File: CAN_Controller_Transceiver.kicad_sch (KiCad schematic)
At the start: 31 parts, among them J11 Screw_Terminal_01x02, J12 DB9_Male, SW1 SW_SPDT, U1 MCP2515-xSO, U2 MCP2551-I-SN, U3 LD1117S50TR_SOT223, Y1 8MHz Crystal

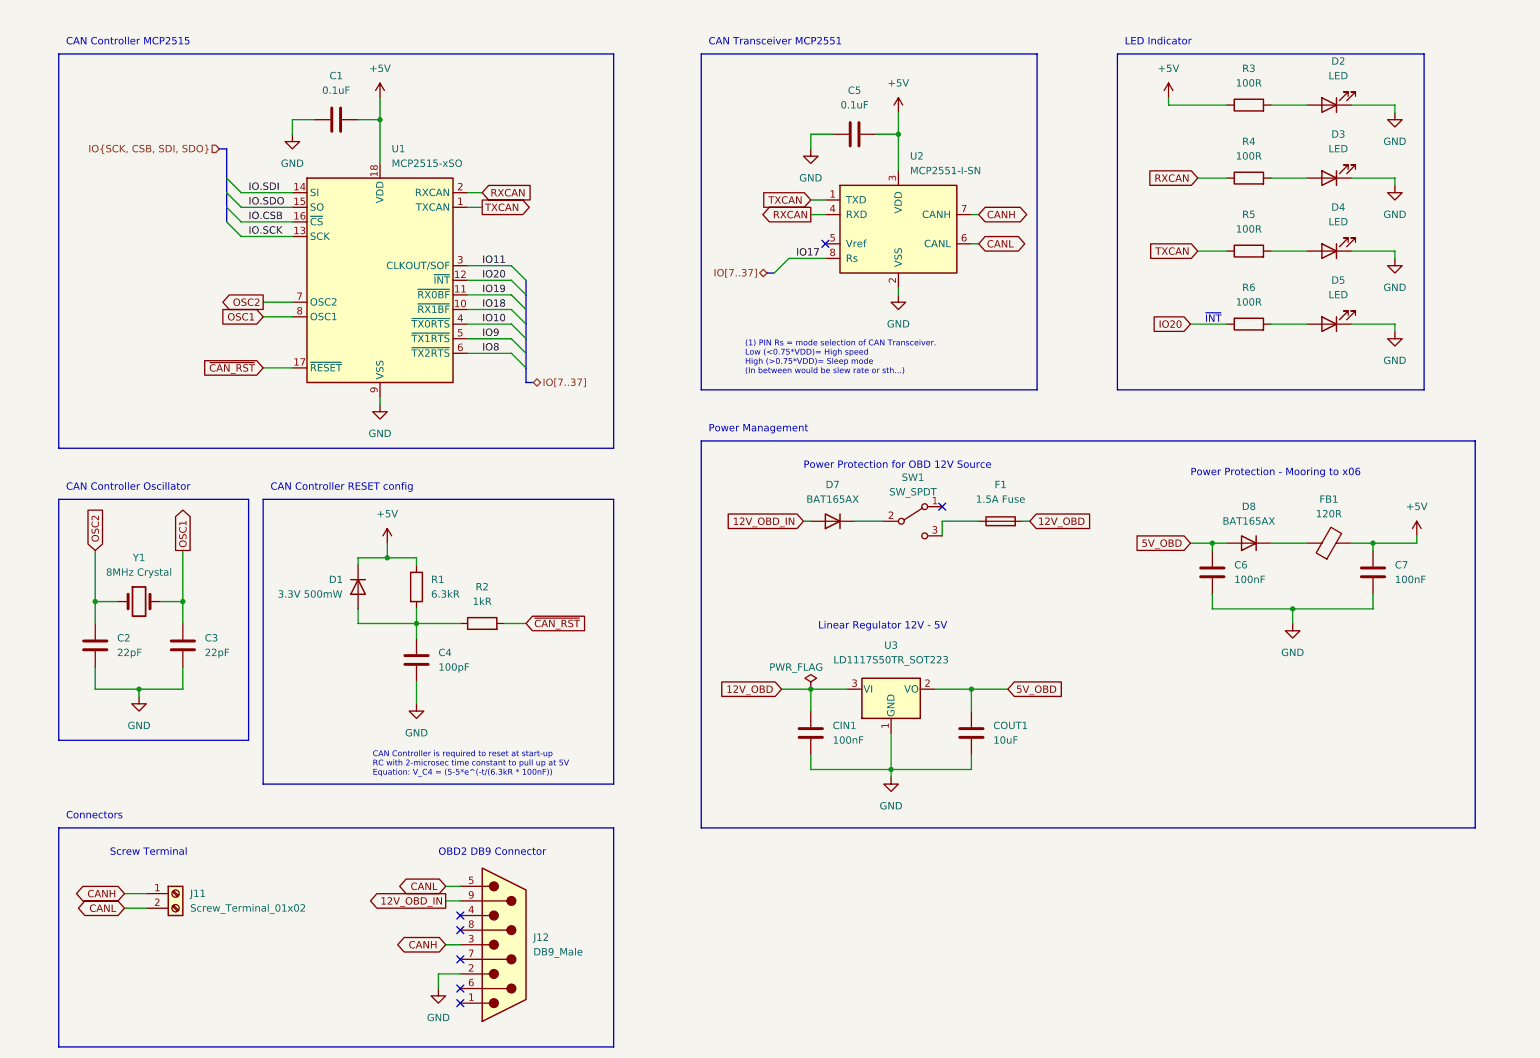
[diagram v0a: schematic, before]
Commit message: Complete board (1)
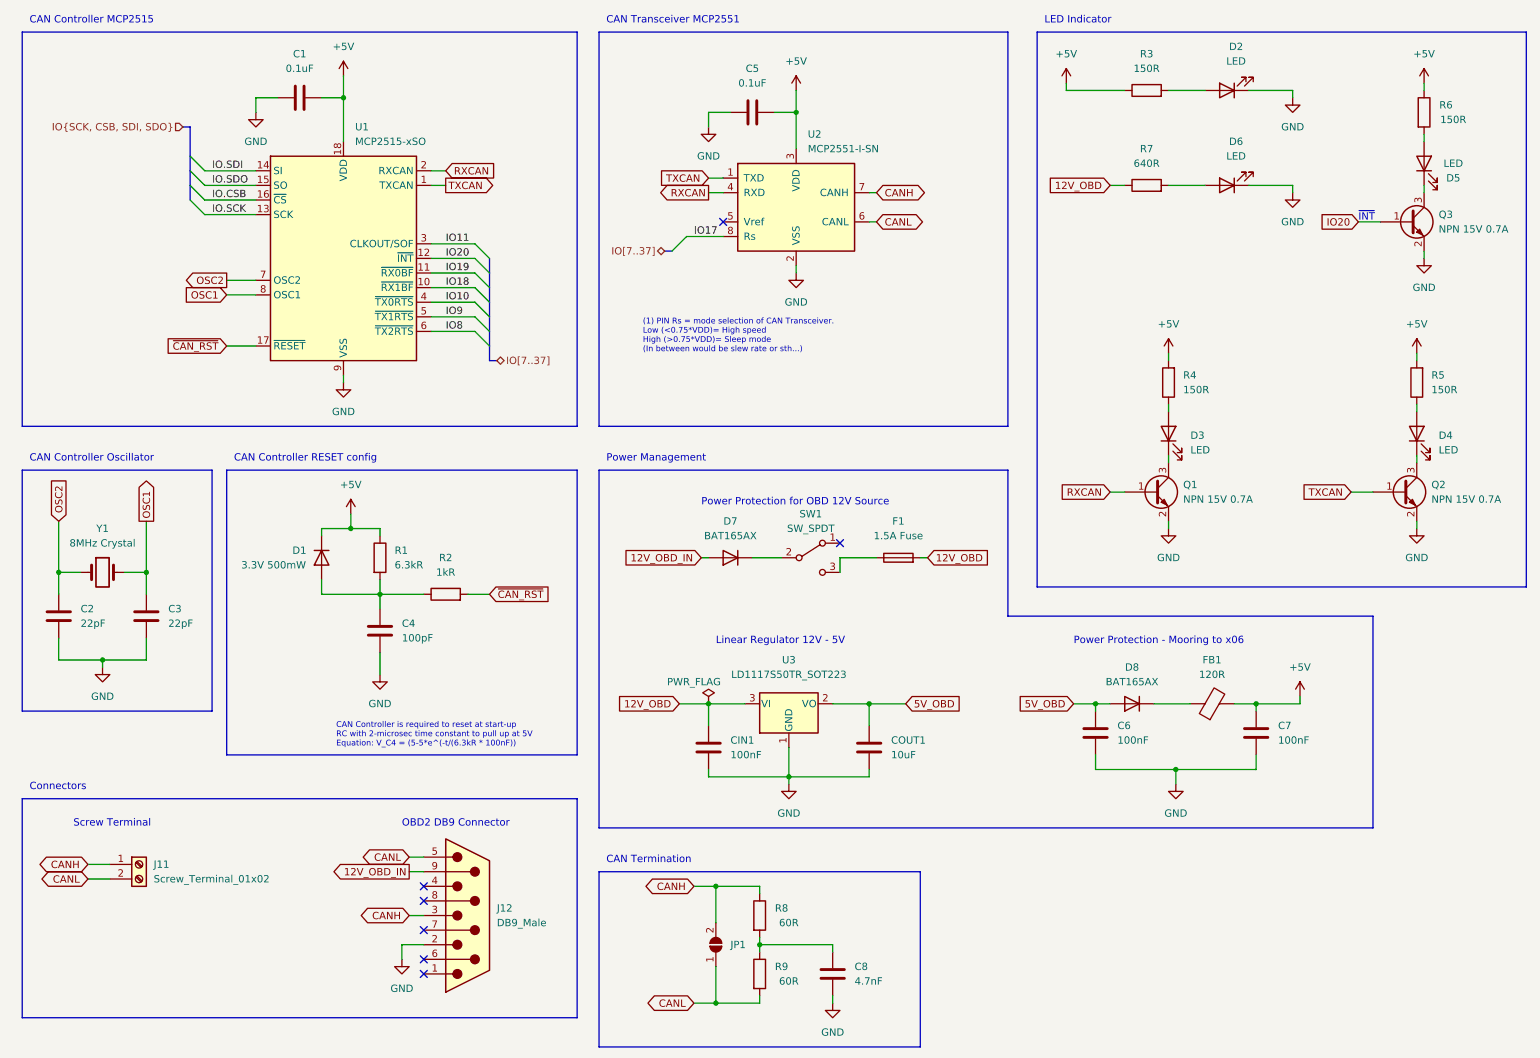
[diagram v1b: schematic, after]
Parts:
- added C8: 4.7nF, Capacitor_SMD:C_0603_1608Metric_Pad1.08x0.95mm_HandSolder, symbol Device:C
- added D6: LED, LED_SMD:LED_0603_1608Metric_Pad1.05x0.95mm_HandSolder, symbol Device:LED
- added JP1: SolderJumper_2_Open, Connector_PinHeader_2.00mm:PinHeader_1x02_P2.00mm_Vertical, symbol Jumper:SolderJumper_2_Open
- added Q1, Q2, Q3: NPN 15V 0.7A, Package_TO_SOT_SMD:SC-59_Handsoldering, symbol Device:Q_NPN_BEC
- added R7: 640R, Resistor_SMD:R_0603_1608Metric_Pad0.98x0.95mm_HandSolder, symbol Device:R
- added R8, R9: 60R, Resistor_SMD:R_0603_1608Metric_Pad0.98x0.95mm_HandSolder, symbol Device:R
- R3, R4, R5, R6: value 100R -> 150R
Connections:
- net +5V: now also R4.2, R5.2, R6.1
- net 12V_OBD: now also R7.1
- net CANH: now also JP1.2 (B), R8.1
- net CANL: now also JP1.1 (A), R9.2
- net GND: now also C8.2, D6.1 (K), Q1.2 (E), Q2.2 (E), Q3.2 (E); no longer D3.1 (K), D4.1 (K), D5.1 (K)
- net IO20: now also Q3.1 (B); no longer R6.1
- net RXCAN: now also Q1.1 (B); no longer R4.1
- net TXCAN: now also Q2.1 (B); no longer R5.1
- net at D3.2 (A): now also R4.1; no longer R4.2
- net at D4.2 (A): now also R5.1; no longer R5.2
- new net: D6.2 (A), R7.2
- new net: C8.1, R8.2, R9.1
- new net: D5.1 (K), Q3.3 (C)
- new net: D3.1 (K), Q1.3 (C)
- new net: D4.1 (K), Q2.3 (C)
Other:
- note added: "CAN Termination"
- moved on the sheet: C1, C2, C3, C4, C5, C6, C7, CIN1, COUT1, D1, D2, D3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
